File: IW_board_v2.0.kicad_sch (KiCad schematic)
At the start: 0 parts

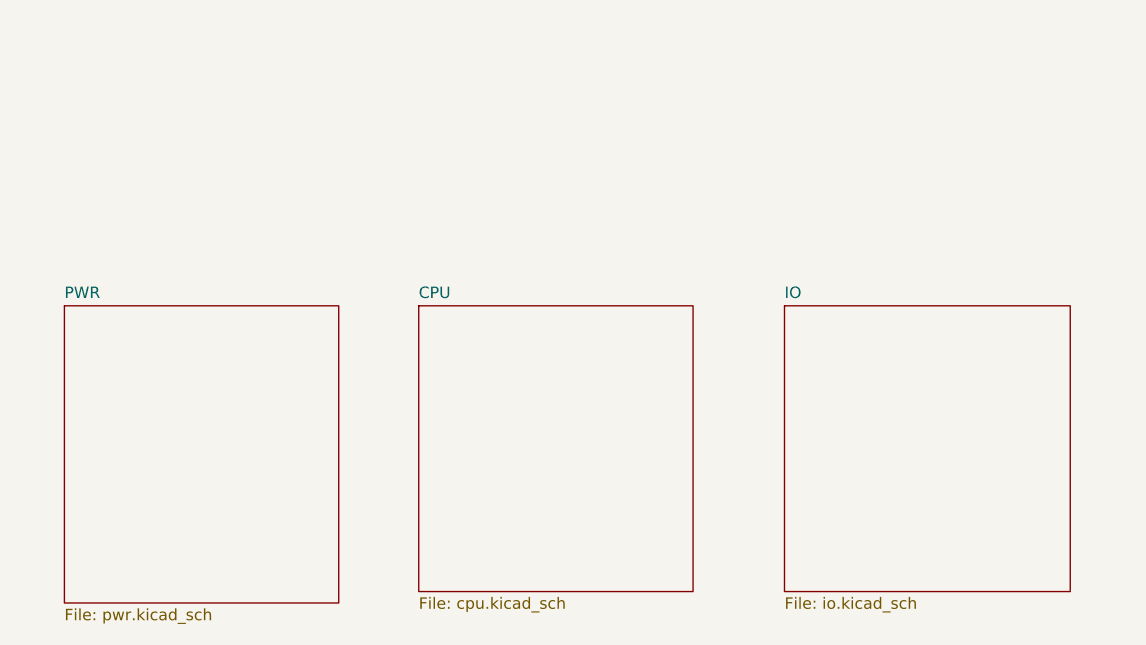
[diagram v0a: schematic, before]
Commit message: Rev 1.0
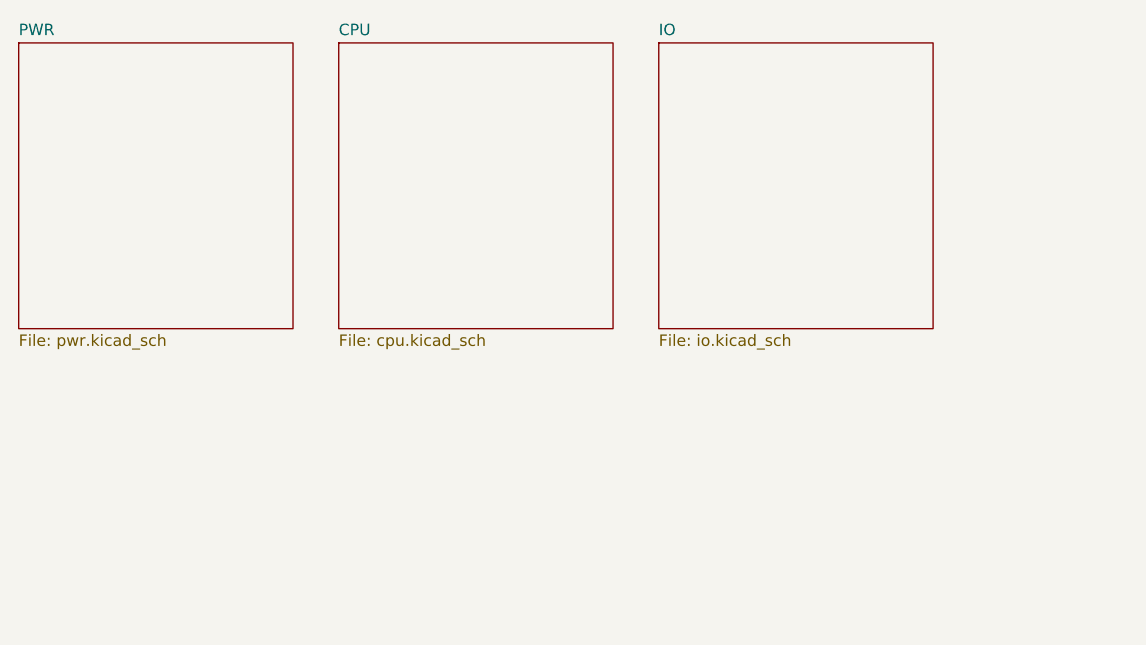
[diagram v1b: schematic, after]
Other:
- title: (none) -> Iron Warriors v2.0 

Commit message: Initial PCB view
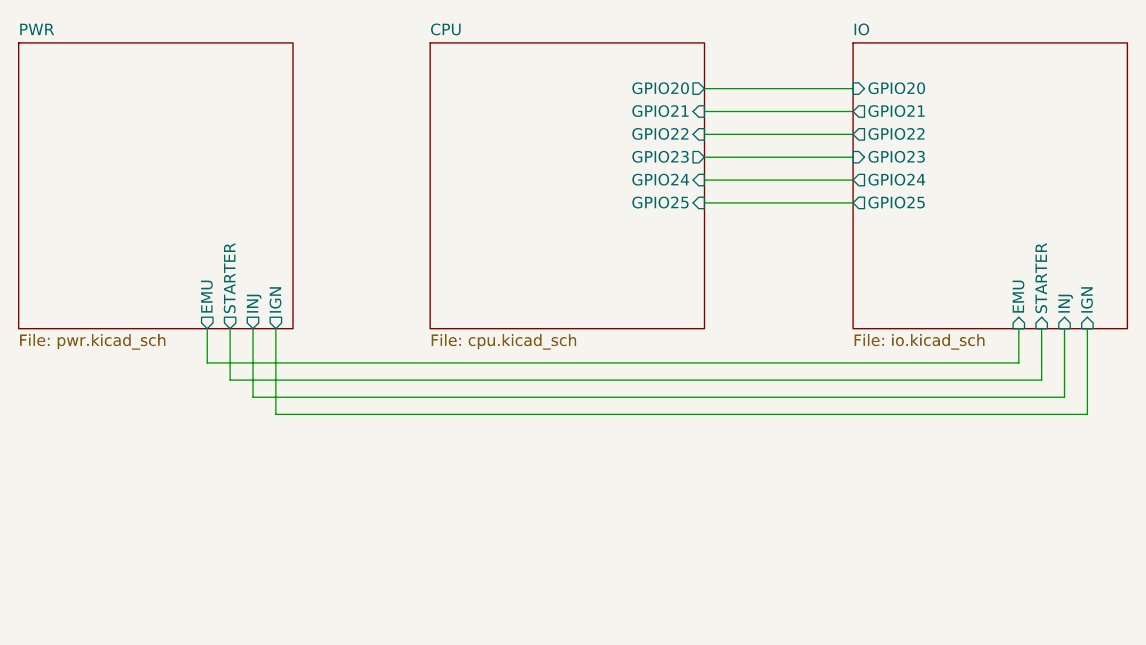
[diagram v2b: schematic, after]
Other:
- sheet CPU ports: added GPIO20, GPIO21, GPIO22, GPIO23, GPIO24, GPIO25; removed none
- sheet IO ports: added EMU, GPIO20, GPIO21, GPIO22, GPIO23, GPIO24, GPIO25, IGN, INJ, STARTER; removed none
- sheet PWR ports: added EMU, IGN, INJ, STARTER; removed none
